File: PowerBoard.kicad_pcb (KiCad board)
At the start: 4 copper layers, 50 x 50 mm, 62 parts, among them Q3 PSMN020-100YS, Q4 PSMN020-100YS, U12 TPS16851VMAR, U13 LM5050-1, U14 TPS16851VMAR, U15 LM5050-1

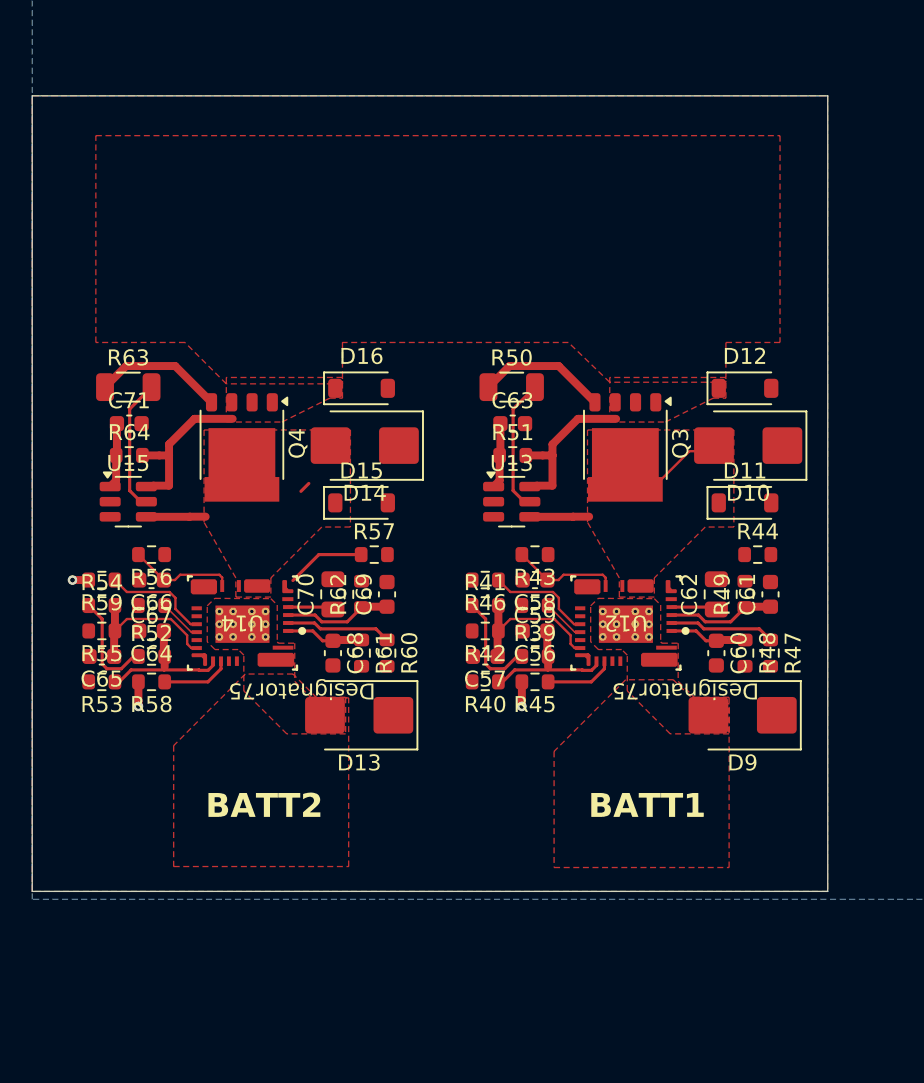
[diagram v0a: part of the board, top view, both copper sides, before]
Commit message: Working on tp
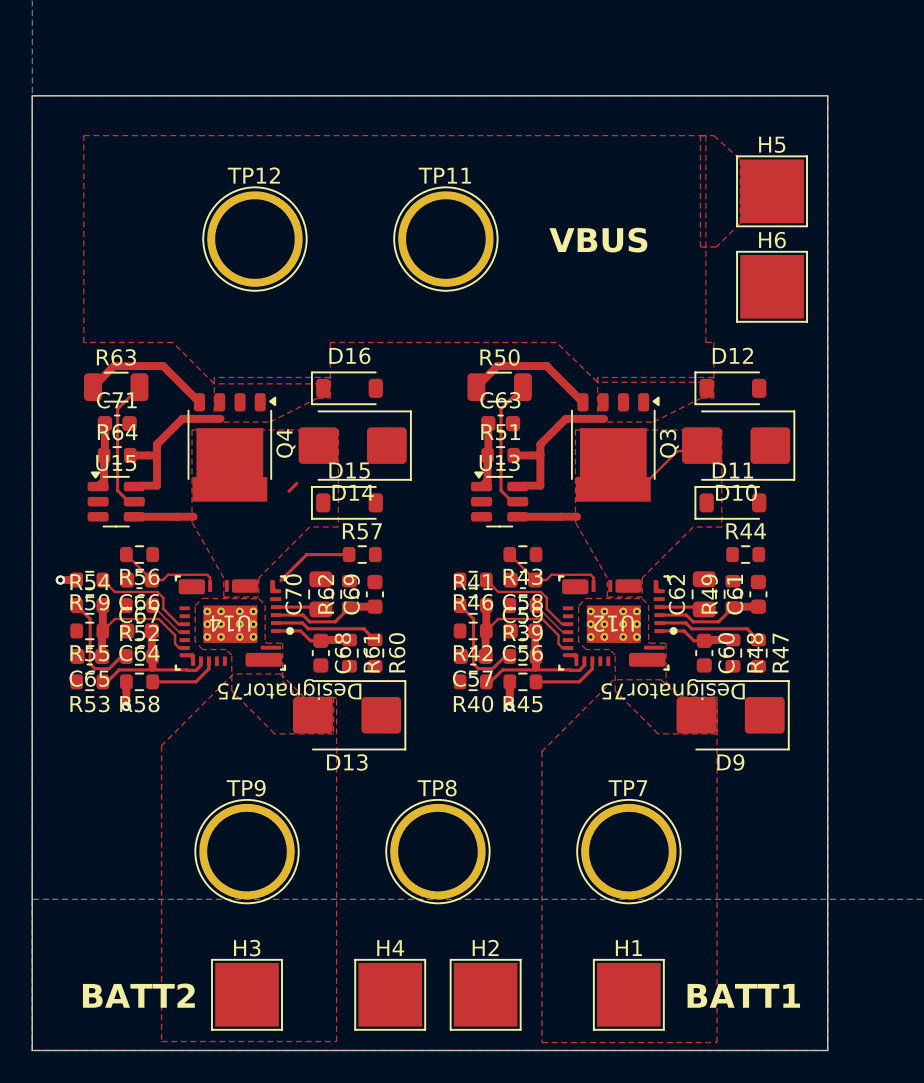
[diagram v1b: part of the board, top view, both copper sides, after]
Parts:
- added H1: MountingHole_Pad_MP, TestPoint:TestPoint_Pad_4.0x4.0mm, F.Cu at (132.5, 151.0)
- added H2: MountingHole_Pad_MP, TestPoint:TestPoint_Pad_4.0x4.0mm, F.Cu at (123.5, 151.0)
- added H3: MountingHole_Pad_MP, TestPoint:TestPoint_Pad_4.0x4.0mm, F.Cu at (108.5, 151.0)
- added H4: MountingHole_Pad_MP, TestPoint:TestPoint_Pad_4.0x4.0mm, F.Cu at (117.5, 151.0)
- added H5: MountingHole_Pad_MP, TestPoint:TestPoint_Pad_4.0x4.0mm, F.Cu at (141.5, 100.5)
- added H6: MountingHole_Pad_MP, TestPoint:TestPoint_Pad_4.0x4.0mm, F.Cu at (141.5, 106.5)
- added TP11: BATT2_DRV_RTN, TestPoint:TestPoint_Plated_Hole_D5.0mm, F.Cu at (121.0, 103.5)
- added TP12: BATT2_DRV_RTN, TestPoint:TestPoint_Plated_Hole_D5.0mm, F.Cu at (109.0, 103.5)
- added TP7: BATT1_DRV_TP, TestPoint:TestPoint_Plated_Hole_D5.0mm, F.Cu at (132.5, 142.0)
- added TP8: BATT1_RTN_TP, TestPoint:TestPoint_Plated_Hole_D5.0mm, F.Cu at (120.5, 142.0)
- added TP9: BATT2_DRV_RTN, TestPoint:TestPoint_Plated_Hole_D5.0mm, F.Cu at (108.5, 142.0)
- moved C60 0.76 mm to (137.2, 129.5)
- moved C61 0.76 mm to (140.6, 125.8)
- moved C62 0.76 mm to (137.2, 125.8)
- moved C63 0.76 mm to (124.4, 115.1)
- moved C64 0.76 mm to (101.7, 128.1)
- moved C65 0.76 mm to (98.6, 129.7)
- moved C66 0.76 mm to (101.7, 124.9)
- moved C67 0.76 mm to (101.7, 126.5)
- moved C68 0.76 mm to (113.1, 129.5)
- moved C70 0.76 mm to (113.1, 125.8)
- moved D10 0.76 mm to (139.2, 116.5)
- moved D11 0.76 mm to (139.0, 120.1)
- moved D12 0.76 mm to (139.0, 112.9)
- moved D14 0.76 mm to (115.1, 116.5)
- moved D15 0.76 mm to (114.9, 120.1)
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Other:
- board size 50 x 50 mm -> 50 x 60 mm
- board text added: "VBUS"
